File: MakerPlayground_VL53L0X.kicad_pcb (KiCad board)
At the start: 2 copper layers, 22.5 x 19.9 mm, 16 parts, among them J1 Connector, Q1 BSS138, Q2 BSS138, U1 VL53L0X, U2 AP2127K-3.3

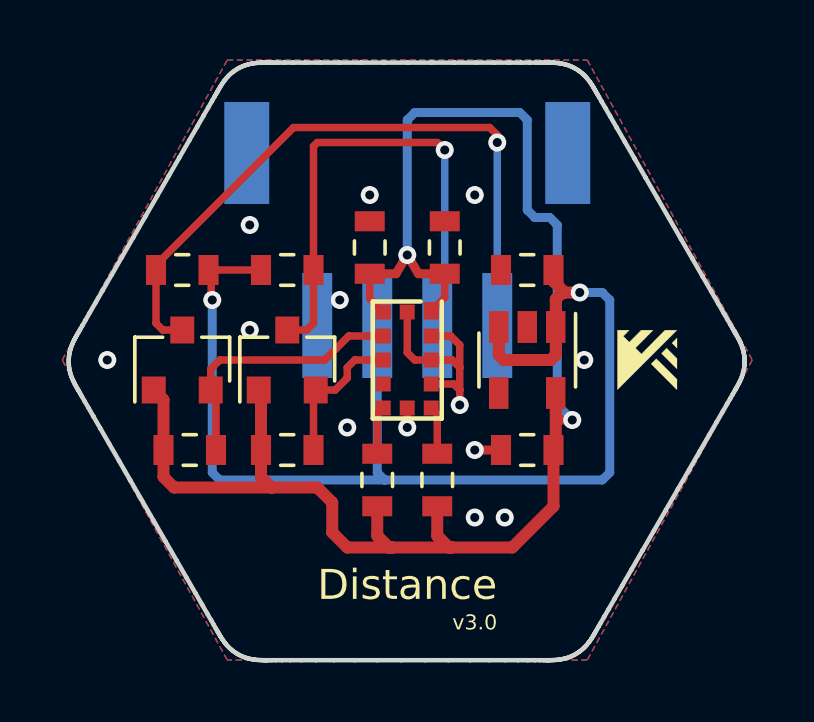
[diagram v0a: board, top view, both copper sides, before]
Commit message: The first commit of MakerPlayground_VL53L0X square shape.
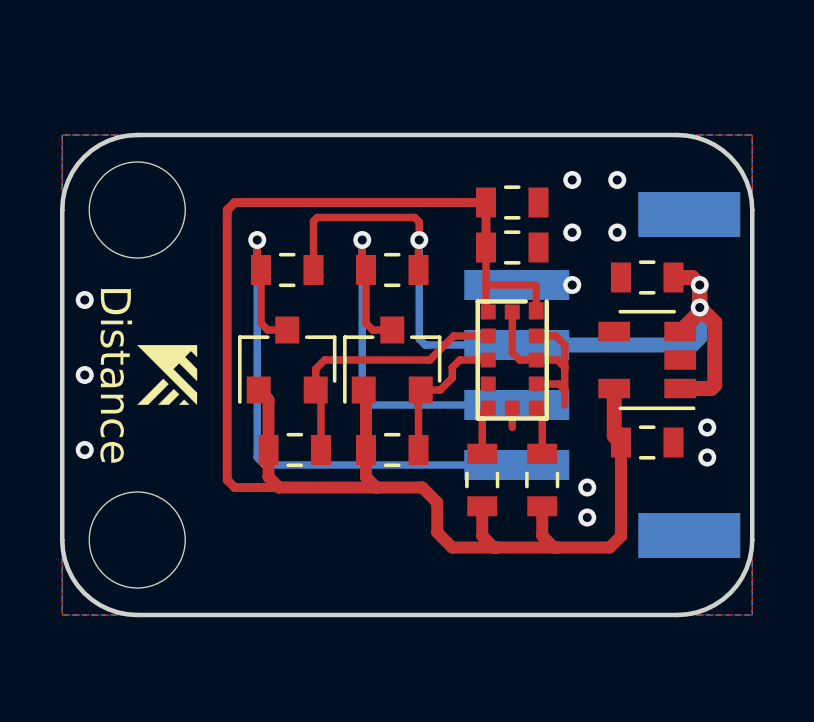
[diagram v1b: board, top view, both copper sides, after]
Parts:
- added REF**: MountingHole_3.2mm_M3, MountingHole:MountingHole_3.2mm_M3, F.Cu at (132.5, 111.0)
- added REF**: MountingHole_3.2mm_M3, MountingHole:MountingHole_3.2mm_M3, F.Cu at (132.5, 100.0)
- moved G*** 16.0 mm to (133.5, 105.5), turned to 270 degrees
- moved J1 7.91 mm to (148.0, 105.5), turned to 270 degrees
- moved C1 4.98 mm to (145.0, 99.8), turned to 0 degrees
- moved C4 4.01 mm to (149.5, 102.2)
- moved C5 4.01 mm to (149.5, 107.8), turned to 0 degrees
- moved U2 4.00 mm to (149.5, 105.0), turned to 180 degrees
- moved Q1 3.50 mm to (141.0, 105.0)
- moved Q2 3.50 mm to (137.5, 105.0)
- moved R1 3.50 mm to (144.0, 109.0)
- moved R2 3.50 mm to (141.0, 102.0), turned to 0 degrees
- moved R3 3.50 mm to (141.0, 108.0)
- moved R4 3.50 mm to (137.5, 102.0)
- moved R5 3.50 mm to (137.8, 108.0)
- moved R6 3.50 mm to (146.0, 109.0)
- moved U1 3.50 mm to (145.0, 105.0)
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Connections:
- J1 pad MP: (no net) -> GND
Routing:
- net VCC: track 40.7 -> 29.0 mm, vias 2 -> 3
- net SDA: track 17.4 -> 14.3 mm
- net SCL: track 22.6 -> 19.8 mm
- net +3V3: track 55.2 -> 54.0 mm, vias 2 -> 0
- net GND: track 8.85 -> 8.06 mm, vias 13 -> 12
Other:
- board size 22.5 x 19.9 mm -> 23 x 16 mm
- board text removed: "v3.0"
